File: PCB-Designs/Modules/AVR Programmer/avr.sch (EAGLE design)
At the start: 21 parts, among them IC1 Atmega8, Q1 12MHZ, X1 MINI-USB_4P-85-32004-10X

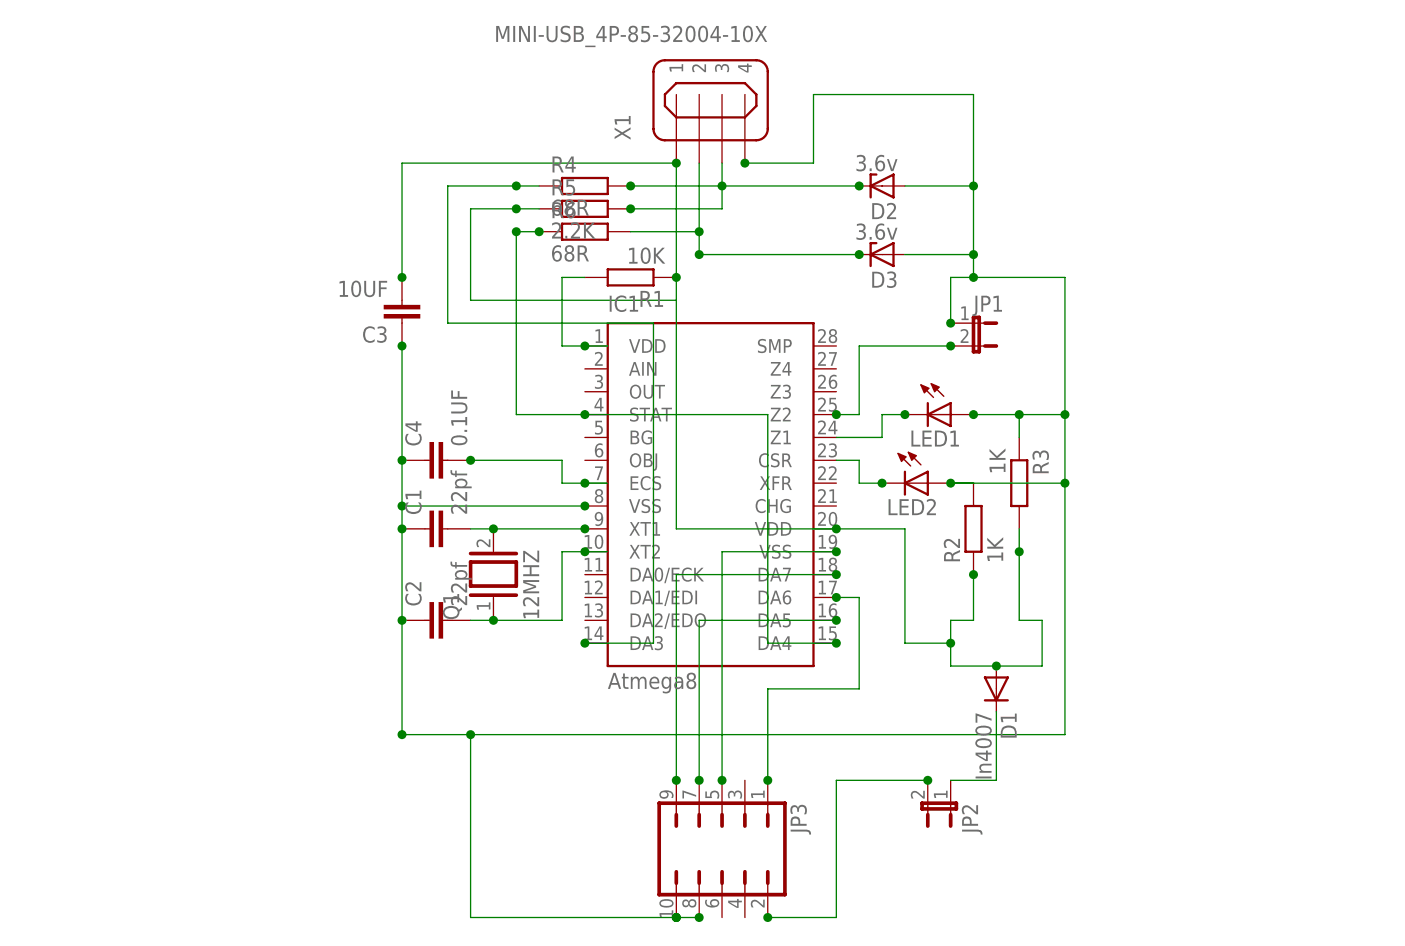
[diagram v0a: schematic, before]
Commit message: new design avr
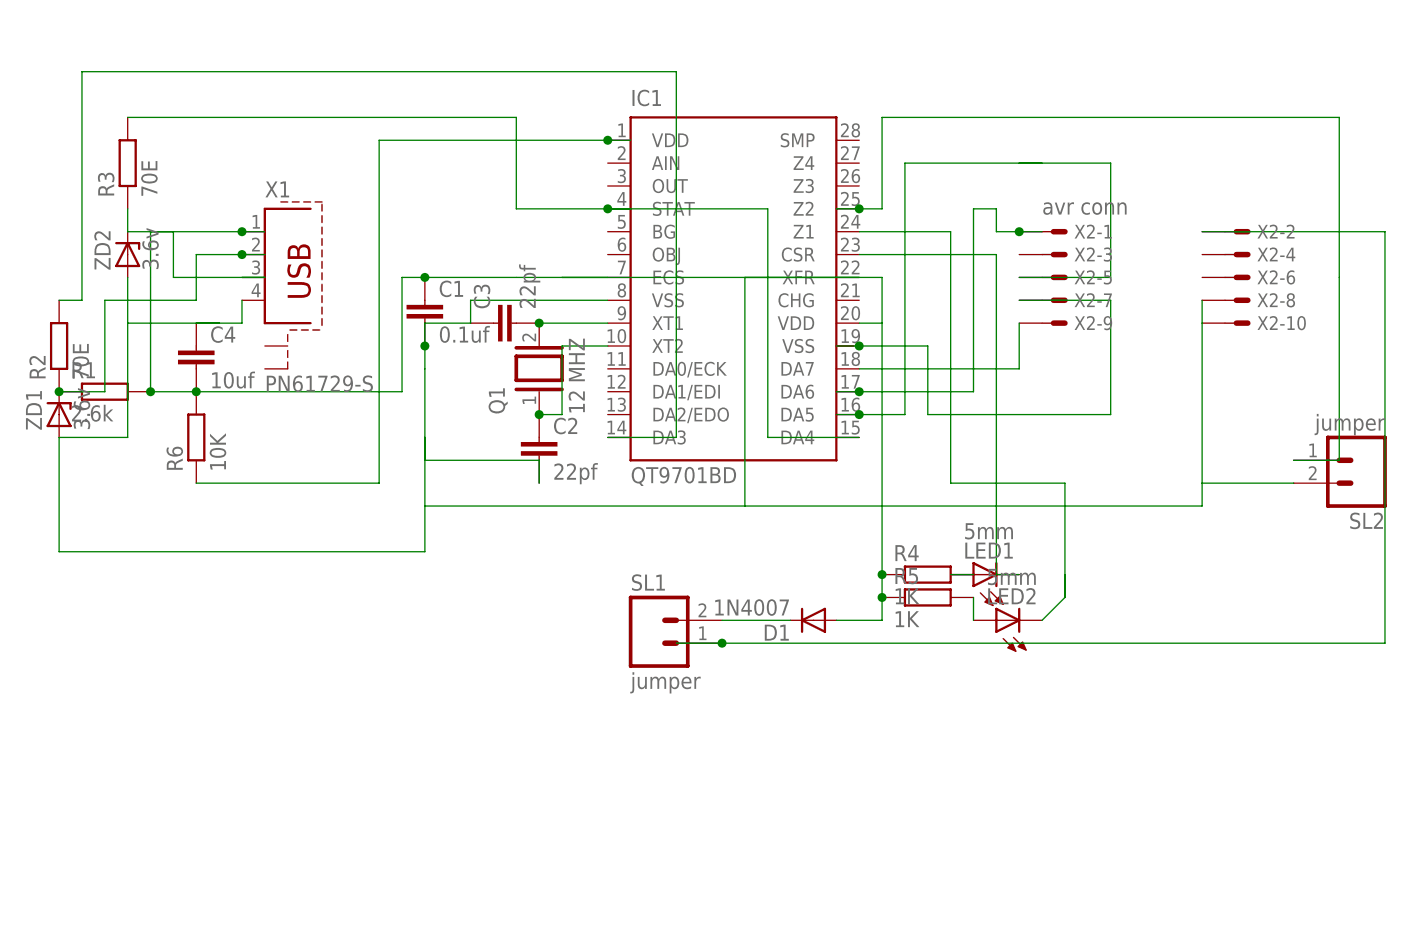
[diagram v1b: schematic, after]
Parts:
- removed D2, D3: 3.6v, diode:1N4728
- removed JP1, JP2: (no value), jumper:JP1E
- removed JP3: (no value), jumper:JP5Q
- added SL1, SL2: jumper, con-amp-quick:M02
- added X2: avr conn, con-panduit:057-010-1
- added ZD1, ZD2: 3.6v, diode:BZD23
- C1: value 22pf -> 0.1uf
- C3: value 10UF -> 22pf
- C4: value 0.1UF -> 10uf
- D1: value In4007 -> 1N4007; device diode:1N5060GP -> diode:1N4004
- IC1: value Atmega8 -> QT9701BD
- LED1, LED2: value (none) -> 5mm; device eagle-ltspice:LED_ELD260 -> led:LED5MM
- Q1: value 12MHZ -> 12 MHZ
- R1: value 10K -> 2.6k; device eagle-ltspice:R0204/7 -> resistor:R-EU_0204/7
- R2, R3: value 1K -> 70E; device eagle-ltspice:R0204/7 -> resistor:R-EU_0204/7
- R4: value 68R -> 1K; device eagle-ltspice:R0204/7 -> resistor:R-EU_0204/7
- R5: value 2.2K -> 1K; device eagle-ltspice:R0204/7 -> resistor:R-EU_0204/7
- R6: value 68R -> 10K; device eagle-ltspice:R0204/7 -> resistor:R-EU_0204/7
- X1: value MINI-USB_4P-85-32004-10X -> PN61729-S; device con-cypressindustries:MINI-USB_4P-85-32004-10X -> con-berg:PN61729-S
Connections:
- removed net N$12: IC1.DA4, IC1.STAT, R6.1
- new net N$20: IC1.Z2, SL2.1
- new net N$21: LED1.A, R4.2
- net N$1: now also C3.2; no longer C1.2
- net N$10: now also IC1.Z1, LED2.C; no longer IC1.DA6, JP3.1
- net N$11: now also D1.C, SL1.2; no longer IC1.DA3, R4.1
- net N$13: now also IC1.CSR, LED1.C; no longer C4.2, IC1.ECS
- net N$14: now also R5.2; no longer C1.1, C2.1, C3.1, C4.1, D2.A, D3.A, IC1.VSS, JP1.1, JP3.10, JP3.8, LED1.A, R2.2, R3.1, X1.4
- net N$15: now also SL1.1, X2-2.S; no longer JP2.2, JP3.2
- net N$16: now also IC1.DA6, X2-1.S; no longer IC1.DA5, JP3.7
- net N$17: now also IC1.DA5, X2-5.S; no longer IC1.VSS@1, JP3.5
- net N$18: now also IC1.VSS@1, X2-7.S; no longer IC1.DA7, JP3.9
- net N$19: now also IC1.DA7, X2-9.S; no longer IC1.VDD, R1.2
- net N$2: now also C2.1; no longer C2.2
- net N$3: now also IC1.VDD, R6.1; no longer D2.C, R4.2, R5.2, X1.3
- net N$4: now also R1.1, R2.1, X1.2, ZD1.C; no longer IC1.CSR, LED2.C
- net N$5: now also C1.2, C2.2, C3.1, C4.1, IC1.VSS, IC1.XFR, SL2.2, X1.4, X2-10.S, X2-8.S, ZD1.A, ZD2.A; no longer IC1.Z1, LED1.C
- net N$6: now also IC1.DA3, R2.2; no longer D3.C, R6.2, X1.2
- net N$7: now also R3.1, X1.3, ZD2.C; no longer C3.2, D1.A, IC1.VDD@1, R1.1, R2.1, R3.2, R5.1, X1.1
- net N$8: now also IC1.DA4, IC1.STAT, R3.2; no longer D1.C, JP2.1
- net N$9: now also C1.1, C4.2, D1.A, IC1.ECS, IC1.VDD@1, R1.2, R4.1, R5.1, R6.2, X1.1; no longer IC1.Z2, JP1.2
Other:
- moved on the sheet: C1, C2, C3, C4, D1, IC1, LED1, LED2, Q1, R1, R2, R3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
